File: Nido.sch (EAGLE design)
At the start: 10 parts, among them K1 HE3621, T1 BC337, U1 BME280

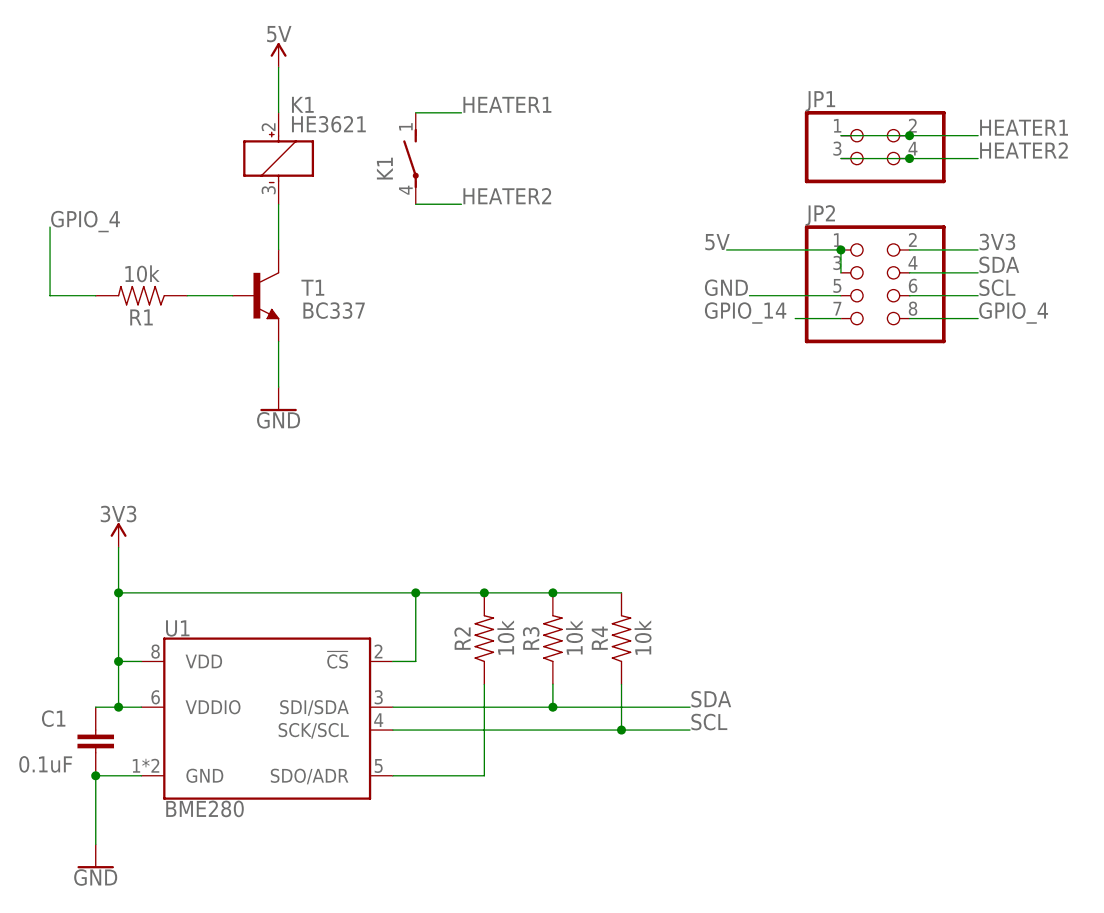
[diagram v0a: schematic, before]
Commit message: Updated Nido PCB v2 files
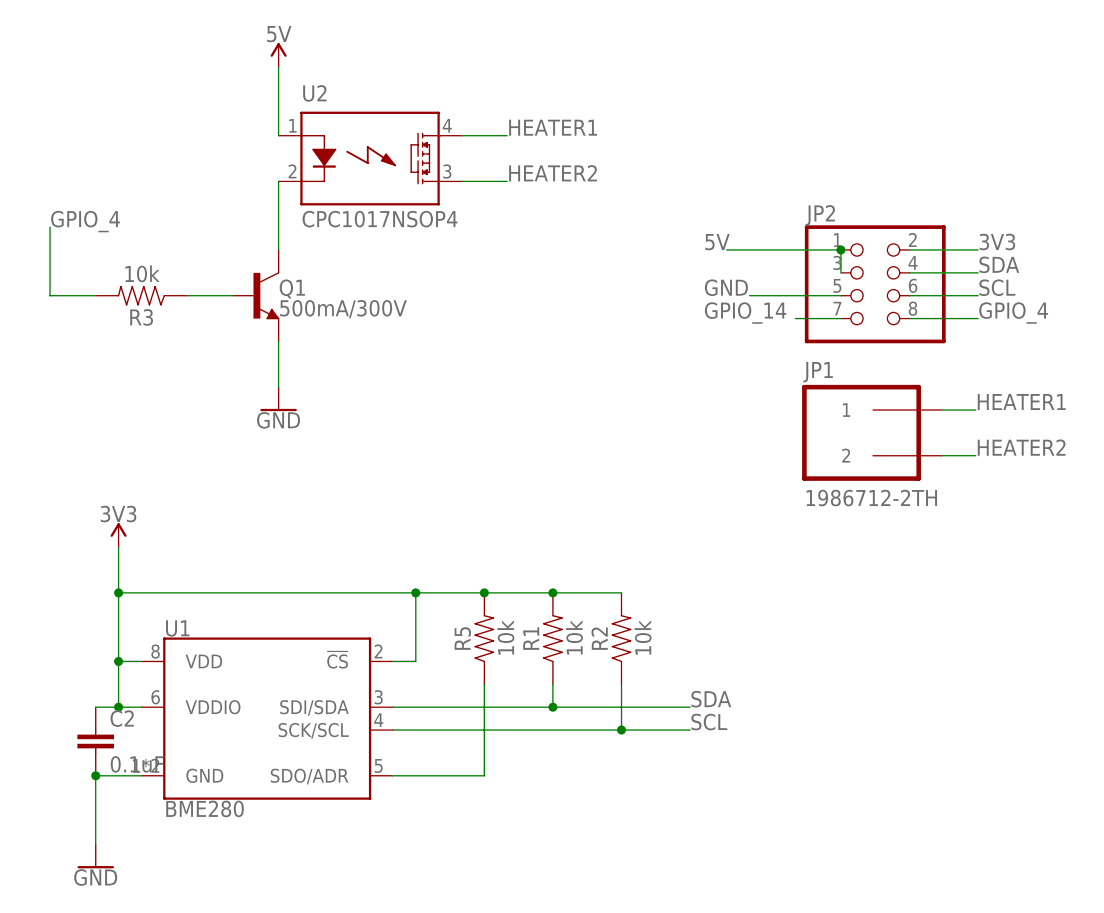
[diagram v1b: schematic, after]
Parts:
- removed C1: 0.1uF, SparkFun-Capacitors:0.1UF-KIT-EZ-50V-20%
- removed K1: HE3621, relay:HE3621
- removed R4: 10k, SparkFun-Resistors:1KOHM-HORIZ-1/4W-1%
- removed T1: BC337, transistor:BC337
- added C2: 0.1uF, SparkFun-Capacitors:0.1UF-0402-16V-10%
- added Q1: 500mA/300V, SparkFun-DiscreteSemi:TRANS_NPN-MMBTA42
- added R5: 10k, SparkFun-Resistors:10KOHM-0402-1/16W-1%
- added U2: CPC1017NSOP4, nido:CPC1017NSOP4
- JP1: value (none) -> 1986712-2TH; device pinhead:PINHD-2X2 -> nido:1986712-2TH
- R1, R2, R3: device SparkFun-Resistors:1KOHM-HORIZ-1/4W-1% -> SparkFun-Resistors:10KOHM-0402-1/16W-1%
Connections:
- net 3V3: now also C2.1, R1.2, R5.2; no longer C1.1, R3.2, R4.2
- net 5V: now also U2.+CONTROL; no longer K11.+
- net GND: now also C2.2, Q1.E; no longer C1.2, T1.E
- net GPIO_4: now also R3.2; no longer R1.2
- net HEATER1: now also U2.LOAD2; no longer JP1.2, K12.S
- net HEATER2: now also JP1.2, U2.LOAD1; no longer JP1.3, JP1.4, K12.P
- net N$1: now also R5.1; no longer R2.1
- net N$5: now also Q1.C, U2.-CONTROL; no longer K11.-, T1.C
- net N$6: now also Q1.B, R3.1; no longer R1.1, T1.B
- net SCL: now also R2.1; no longer R4.1
- net SDA: now also R1.1; no longer R3.1
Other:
- moved on the sheet: R1, R2, R3
